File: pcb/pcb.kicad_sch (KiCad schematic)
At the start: 97 parts, among them J1 MJ-4PP-9, J2 MJ-4PP-9, J3 USB_C_Receptacle_USB2.0_16P, SW1 KEY_SW, SW10 KEY_SW, SW11 KEY_SW, SW12 KEY_SW, SW13 KEY_SW, SW14 KEY_SW, SW15 KEY_SW, SW16 KEY_SW, SW17 KEY_SW, SW18 KEY_SW, SW19 KEY_SW, SW2 KEY_SW, SW20 KEY_SW, SW21 KEY_SW, SW22 KEY_SW, SW23 KEY_SW, SW24 KEY_SW, SW25 KEY_SW, SW26 KEY_SW, SW27 RotaryEncoder, SW3 KEY_SW, SW30 KEY_SW, SW31 KEY_SW, SW32 KEY_SW, SW33 KEY_SW, SW34 KEY_SW, SW35 KEY_SW, SW36 KEY_SW, SW37 KEY_SW, SW38 KEY_SW, SW39 KEY_SW, SW4 KEY_SW, SW40 KEY_SW, SW41 KEY_SW, SW42 KEY_SW, SW43 KEY_SW, SW44 KEY_SW, SW45 KEY_SW, SW46 KEY_SW, SW47 KEY_SW, SW48 KEY_SW, SW49 KEY_SW, SW5 KEY_SW, SW50 KEY_SW, SW51 KEY_SW, SW52 KEY_SW, SW53 KEY_SW, SW54 KEY_SW, SW55 RotaryEncoder, SW6 KEY_SW, SW60 RESET_SW, SW61 BOOT_SW, SW7 KEY_SW, SW8 KEY_SW, SW9 KEY_SW, U1 ESP32-S3-WROOM-1, U2 TPS1117LV33S, U3 USBLC6-2SC6

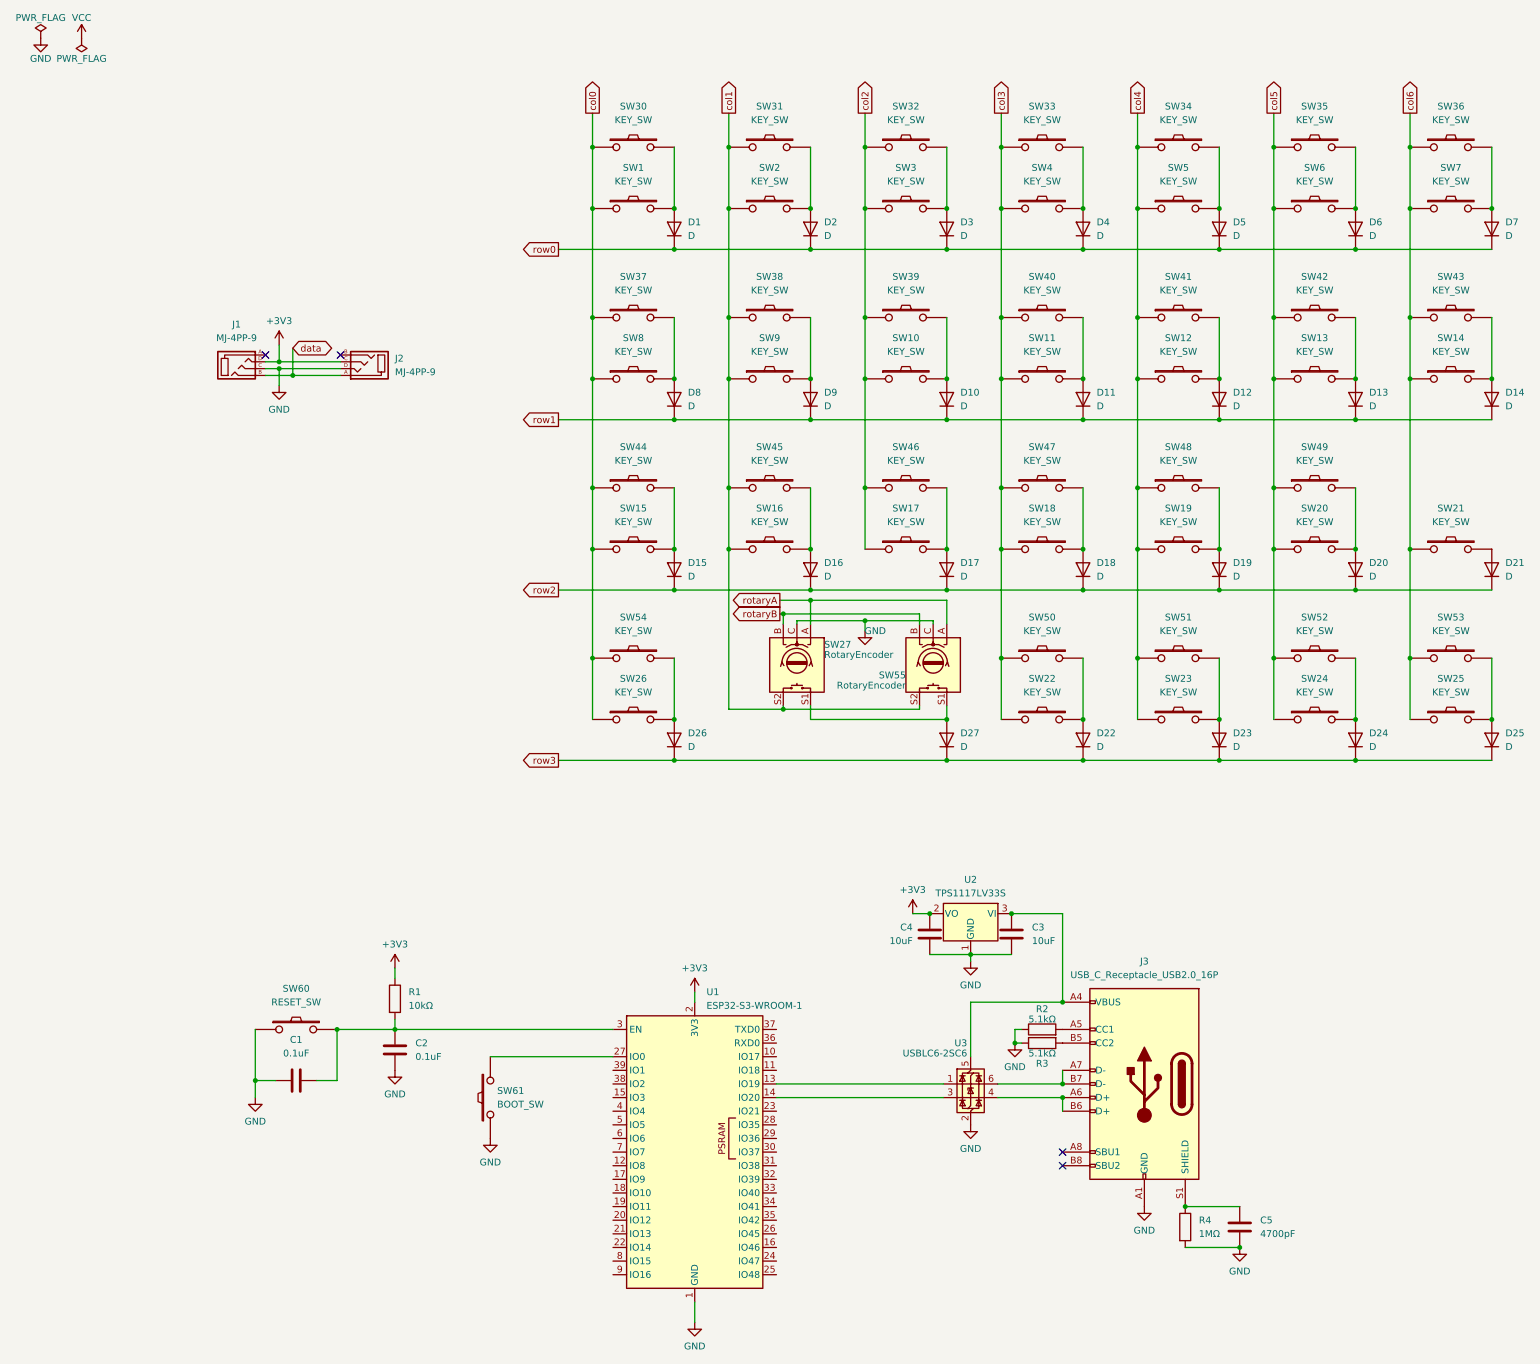
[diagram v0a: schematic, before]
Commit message: split connector close #8
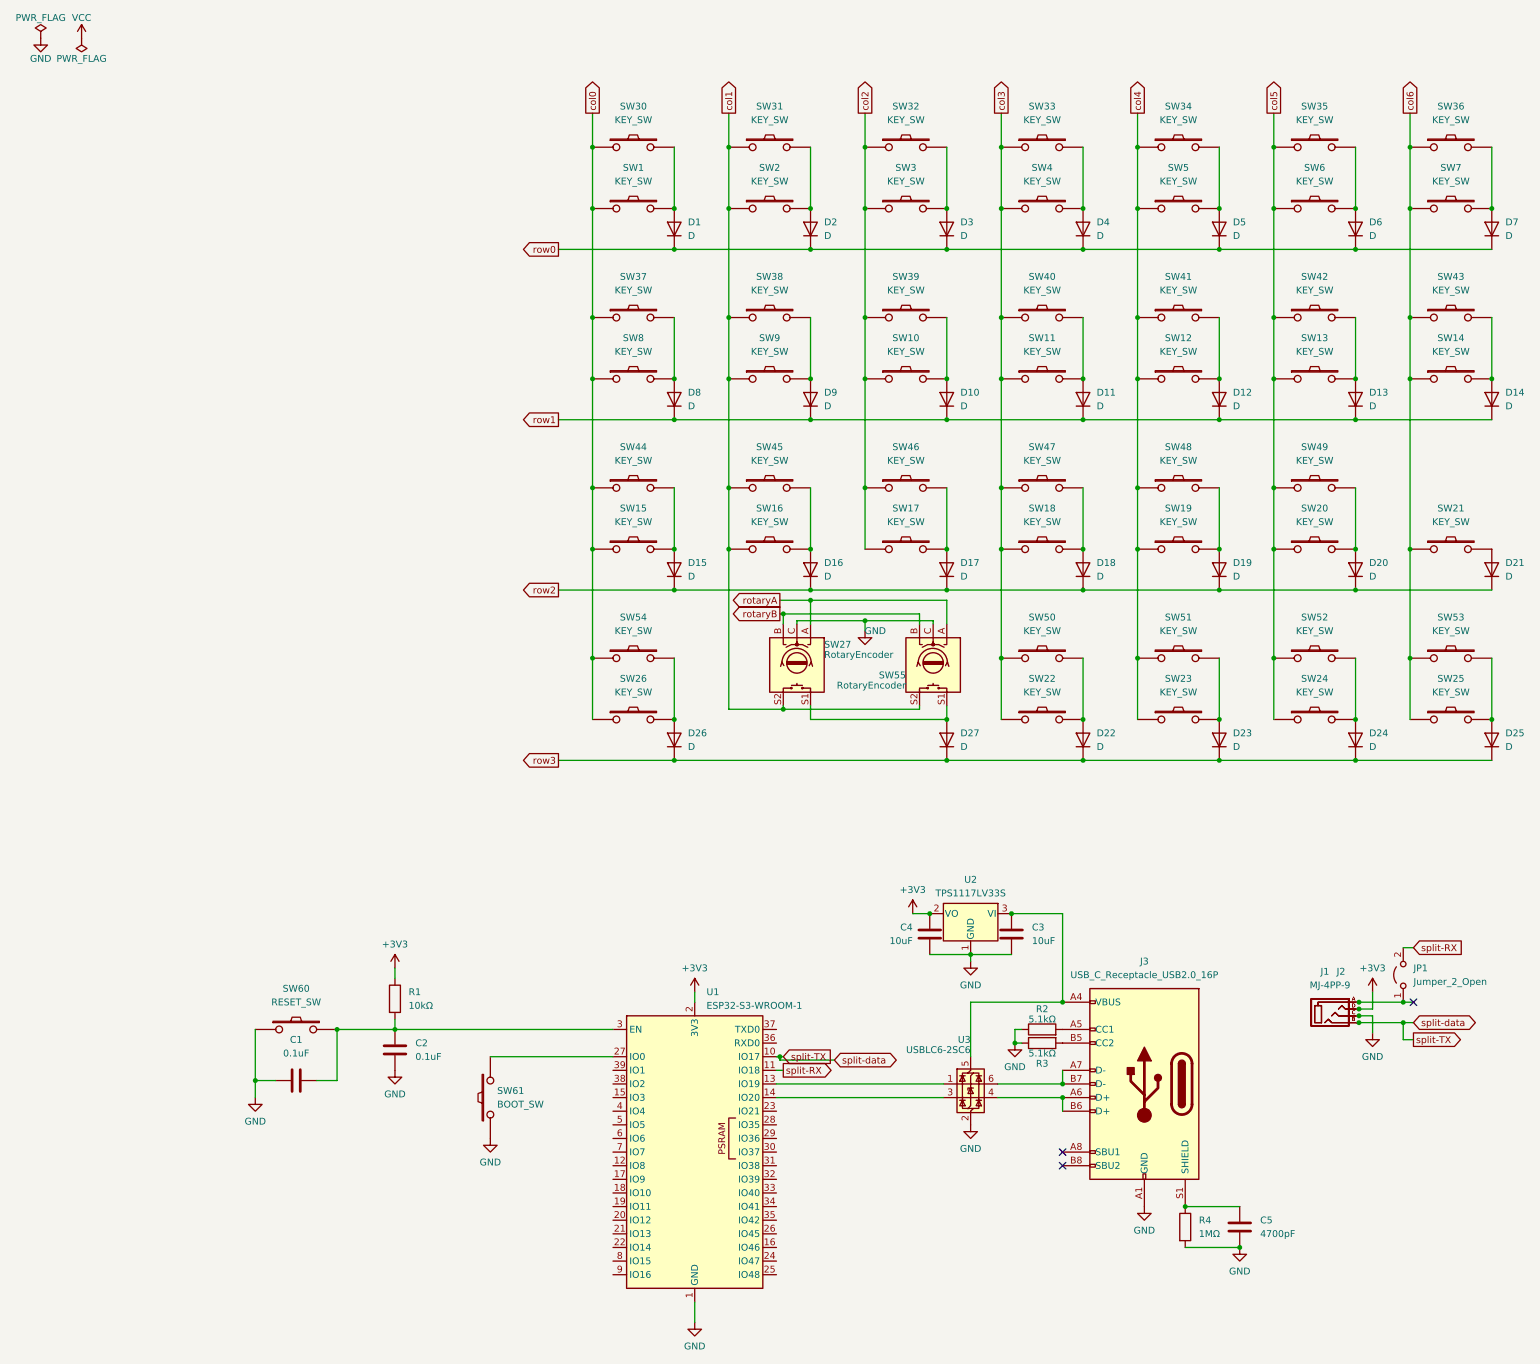
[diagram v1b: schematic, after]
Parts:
- added JP1: Jumper_2_Open, symbol Jumper:Jumper_2_Open
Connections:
- net +3V3: now also J2.D; no longer J2.C
- net GND: now also J2.C; no longer J2.D
- net at J1.A: now also J2.A, JP1.1 (A)
- net split-TX: now reaches J2.B
- net split-TX: now also J1.B, U1.10 (IO17)
- net split-RX: now reaches U1.11 (IO18)
- net split-RX: now also JP1.2 (B)
- removed net data: J1.B, J2.A
- no-connect marks 4 -> 3
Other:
- moved on the sheet: J1, J2
